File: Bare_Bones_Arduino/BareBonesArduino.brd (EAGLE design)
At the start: 43.2 x 61 mm, 15 parts, among them U1 ATMEGA328P_PDIP

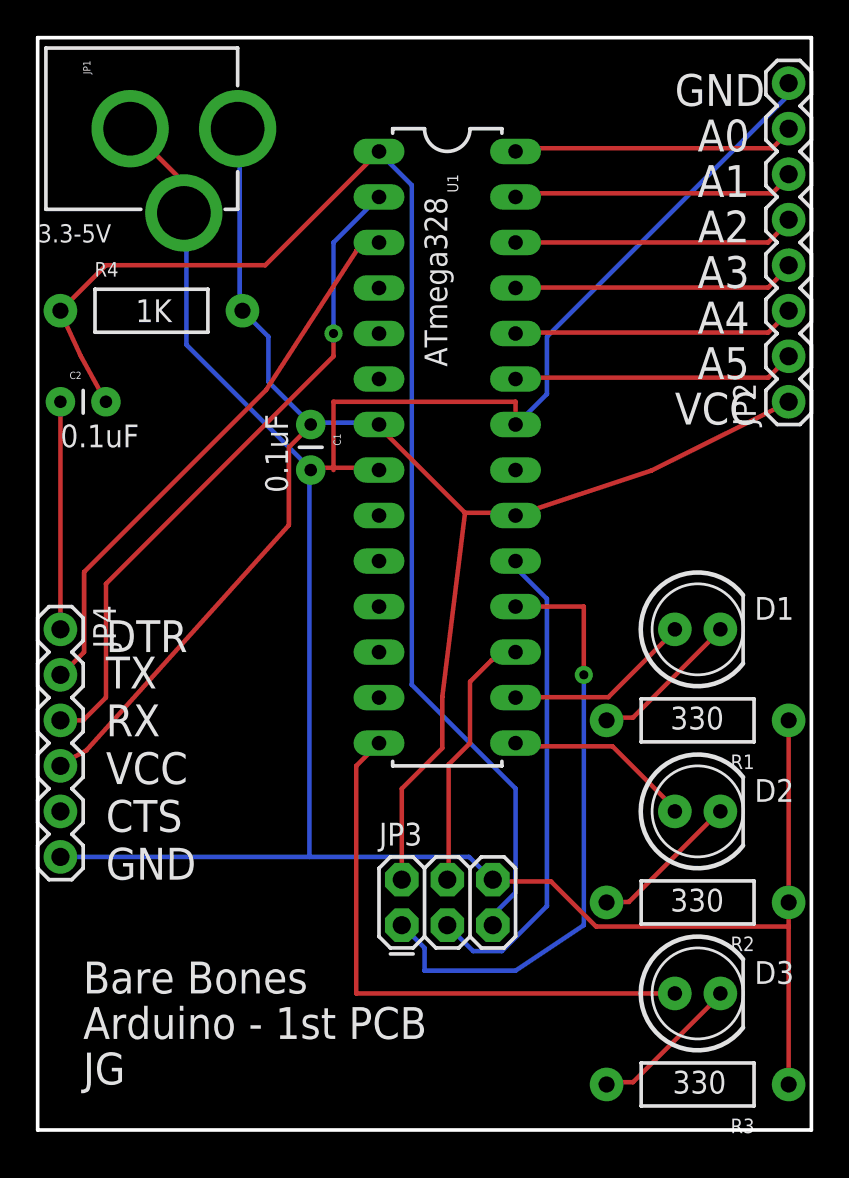
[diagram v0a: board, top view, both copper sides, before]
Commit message: Version 2 smaller design
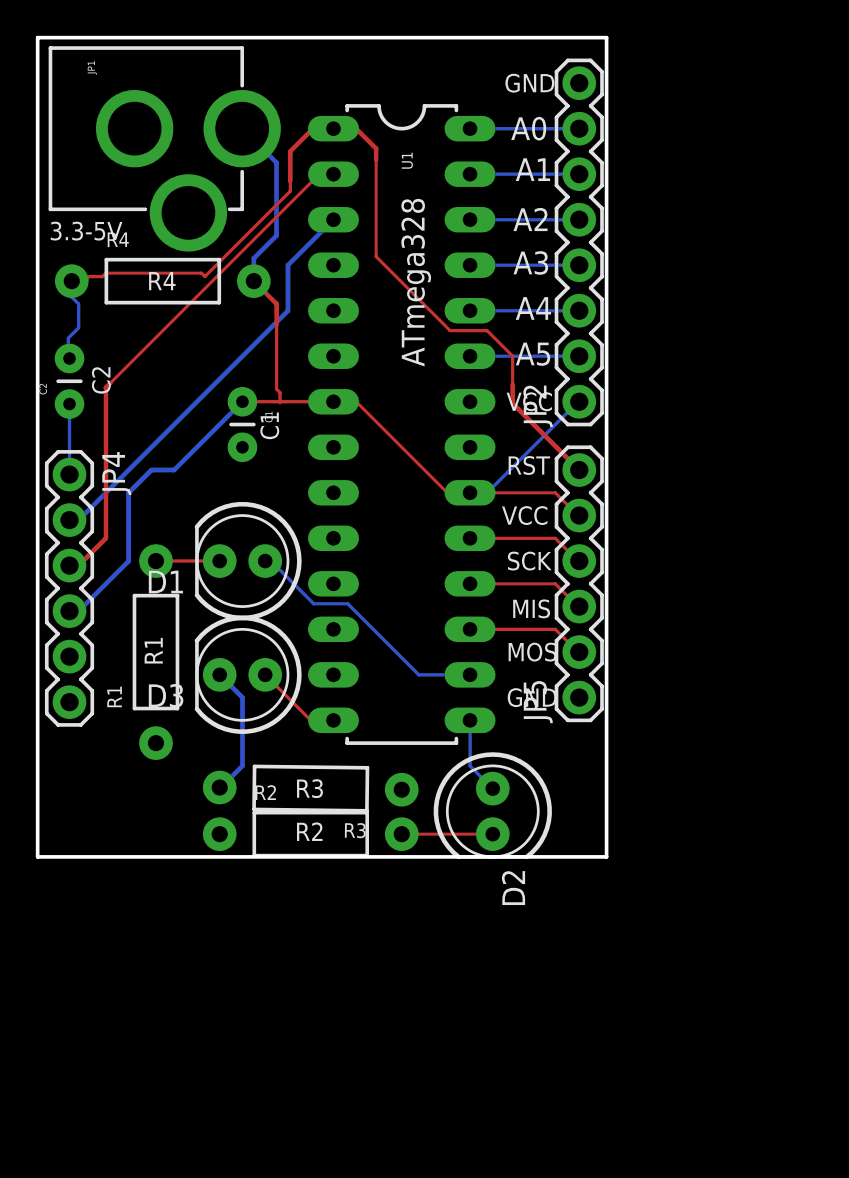
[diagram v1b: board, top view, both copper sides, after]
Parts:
- removed JP3: AVR_SPI_PRG_6PTH, SparkFun-Connectors:2X3
- added JP5: (no value), SparkFun-Connectors:1X06
- moved D3 31.0 mm to (15.2, 44.5), turned to 180 degrees
- moved R1 30.5 mm to (10.4, 45.7), turned to 90 degrees
- moved R3 27.2 mm to (19.1, 38.1), turned to 179.3 degrees
- moved D1 25.7 mm to (15.2, 50.8), turned to 180 degrees
- moved R2 21.9 mm to (19.1, 35.6), turned to 0 degrees
- moved JP2 11.7 mm to (34.0, 59.7)
- moved D2 11.4 mm to (29.2, 36.8), turned to 270 degrees
- moved JP4 8.65 mm to (5.59, 55.6)
- moved C1 4.02 mm to (15.2, 59.7)
- moved U1 2.84 mm to (24.1, 58.4)
- moved R4 1.77 mm to (10.8, 66.4)
- moved C2 0.52 mm to (5.59, 59.6), turned to 90 degrees
- moved JP1 0.25 mm to (1.52, 74.9)
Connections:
- net GND: now also JP5.1; no longer JP3.6
- net MISO: now also JP5.3; no longer JP3.1
- net MOSI: now also JP5.2; no longer JP3.4
- net RESET: now also JP5.6; no longer JP3.5
- net SCK: now also JP5.4; no longer JP3.3
- net VCC: now also JP5.5; no longer JP3.2
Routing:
- net GND: track 152.0 -> 0.00 mm
- net VCC: track 94.9 -> 63.7 mm
- net MISO: track 34.3 -> 6.62 mm, vias 1 -> 0
- net N$5: track 32.3 -> 4.86 mm
- net RESET: track 74.0 -> 51.1 mm
- net SCK: track 27.2 -> 6.62 mm
- net N$13: track 15.9 -> 6.10 mm
- net N$12: track 15.9 -> 6.10 mm
- net N$11: track 15.8 -> 6.10 mm
- net N$10: track 15.8 -> 6.10 mm
- net N$9: track 15.8 -> 6.10 mm
- net N$8: track 15.8 -> 6.10 mm
- net DTR: track 12.7 -> 3.94 mm
- net RX: track 37.3 -> 28.7 mm, vias 1 -> 0
- net TX: track 31.4 -> 23.2 mm
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- added copper zone on layer 16, net GND
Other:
- board size 43.2 x 61 mm -> 31.8 x 45.7 mm
- board text added: "C1"
- board text added: "C2"
- board text added: "MIS"
- board text added: "MOS"
- board text added: "R1"
- board text added: "R2"
- board text added: "R3"
- board text added: "R4"
- board text added: "RST"
- board text added: "SCK"
- board text removed: "0.1uF"
- board text removed: "1K"
- board text removed: "330"
- board text removed: "Arduino - 1st PCB"
- board text removed: "Bare Bones"
- board text removed: "DTR"
- board text removed: "JG"
- board text removed: "TX RX VCC CTS GND"
